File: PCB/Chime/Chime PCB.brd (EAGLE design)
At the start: 99 x 78.9 mm, 33 parts, among them U1 MS5803-02BA, X4 BQ24074

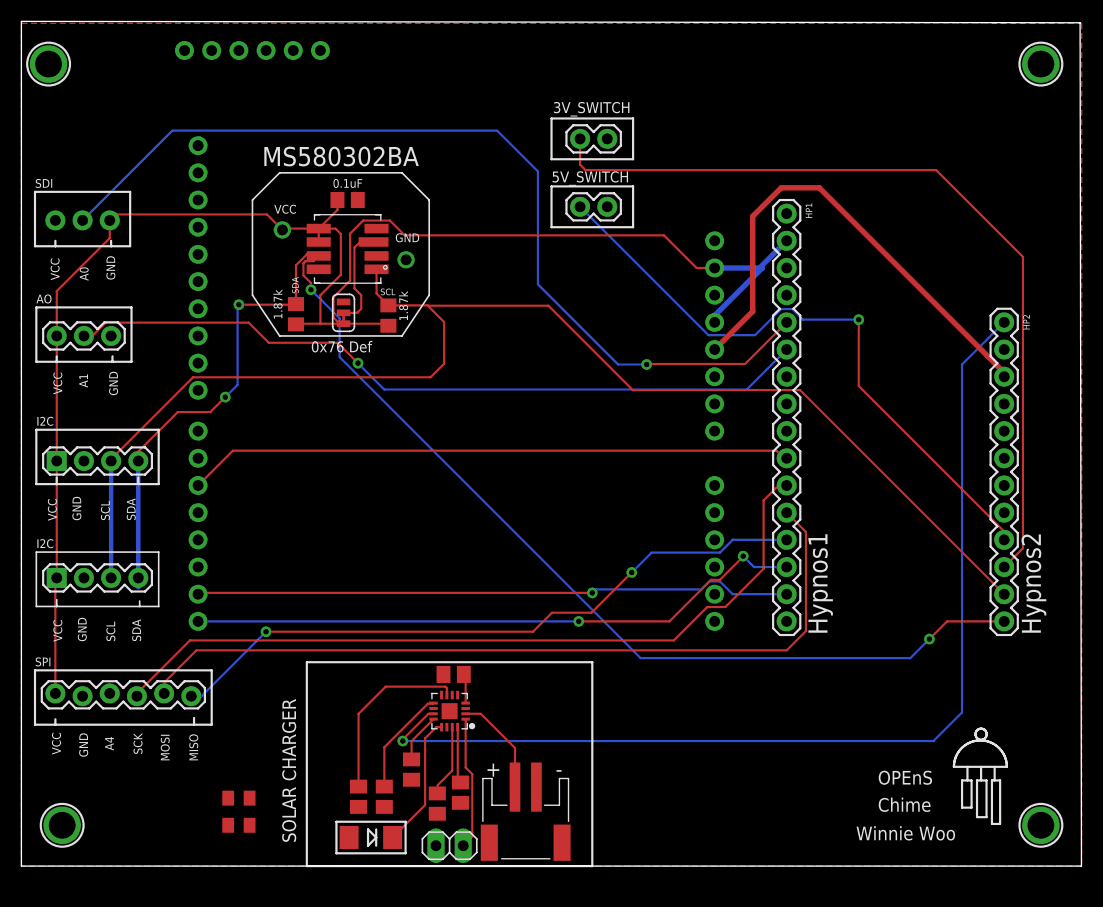
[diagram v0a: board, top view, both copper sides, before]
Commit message: Add files via upload
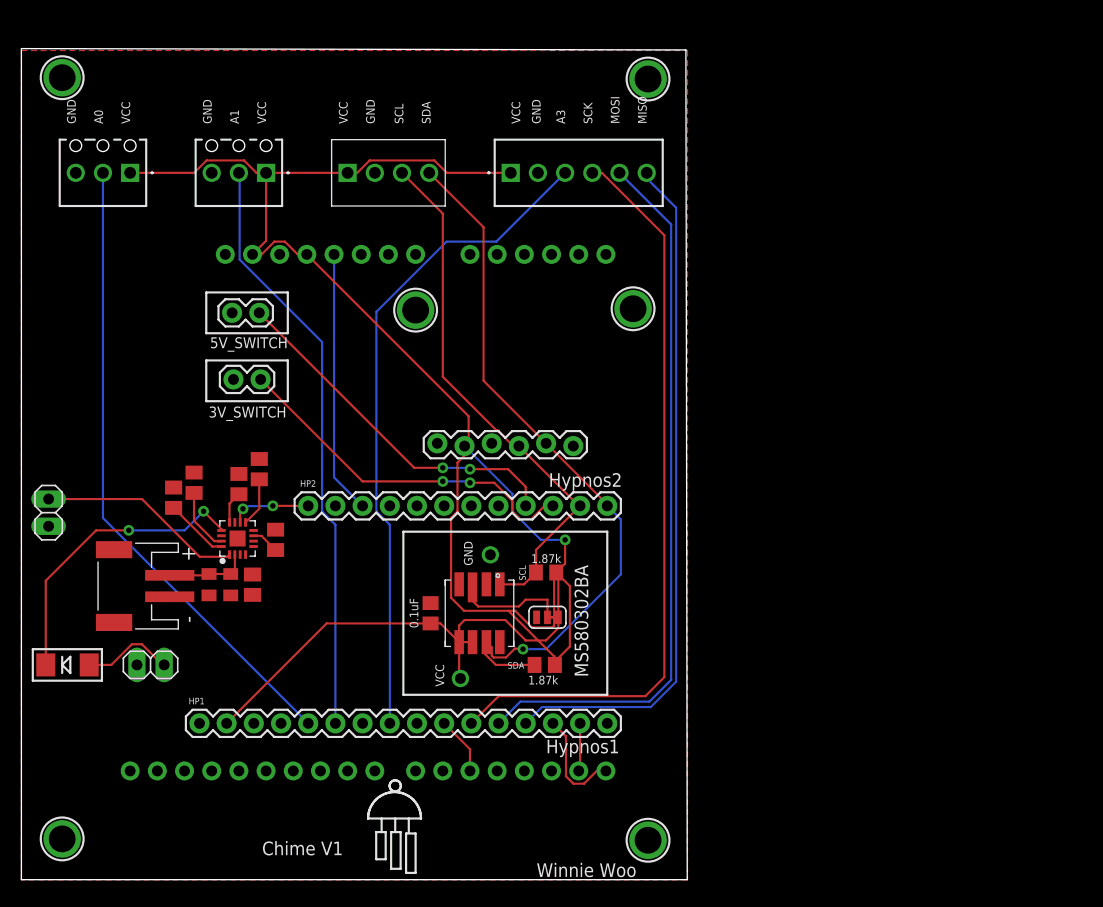
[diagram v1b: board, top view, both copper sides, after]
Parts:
- removed J1_I2C: (no value), SparkFun-Connectors:1X04
- removed J3_AO, J4_SD1: (no value), SparkFun-Connectors:1X03
- removed J6_SPI: (no value), SparkFun-Connectors:1X06_LOCK
- added J1_SPI: 1725698, 1725698:1725698
- added J4_A1, J5_A0: 1725669, 1725669:1725669
- added J6_TSL2591: (no value), SparkFun-Connectors:1X06_LOCK
- added JP9: (no value), pinhead:1X02
- added U$17, U$19: MOUNTINGHOLE2.5, microbuilder:MOUNTINGHOLE_2.5_PLATED
- J2_I2C: value (none) -> 1725672; device SparkFun-Connectors:1X04 -> 1725672:1725672
- U$1: device LTE_BOARD:LTE_BOARD_FOOTPRINT -> LTE_BOARD_LOOM:LTE_BOARD_FOOTPRINT
- moved HP1 72.7 mm to (16.6, 14.6), turned to 0 degrees
- moved HP2 67.2 mm to (26.8, 34.9), turned to 0 degrees
- moved JP8 48.7 mm to (2.54, 34.3), turned to 270 degrees
- moved U$1 45.7 mm to (19.1, 58.4), turned to 180 degrees
- moved JP4 45.1 mm to (41.0, 18.8), turned to 90 degrees
- moved BATT 43.3 mm to (10.2, 27.4), turned to 90 degrees
- moved R1 40.2 mm to (48.9, 20.1), turned to 0 degrees
- moved C1 39.4 mm to (38.2, 24.9), turned to 90 degrees
- moved R9 38.4 mm to (14.2, 35.7), turned to 90 degrees
- moved J2_I2C 38.3 mm to (30.5, 66.0)
- moved R4 37.6 mm to (16.1, 37.1), turned to 90 degrees
- moved J7_S3V 37.4 mm to (22.4, 46.7), turned to 180 degrees
- moved U$4 36.7 mm to (58.5, 74.8)
- moved U$5 36.7 mm to (58.5, 3.68)
- moved U1 36.2 mm to (42.8, 24.9), turned to 90 degrees
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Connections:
- removed net A4: J6_SPI.3
- new net INT: J6_TSL2591.6
- new net VIN: J6_TSL2591.1
- net A0: now also J5_A0.2; no longer J4_SD1.2
- net A1: now also J4_A1.2; no longer J3_AO.2
- net A3: now also J1_SPI.3
- net CHARGER_IN: now also JP9.1
- net GND: now also C5.2, C6.2, J1_SPI.2, J4_A1.3, J5_A0.3, J6_TSL2591.3; no longer J1_I2C.2, J3_AO.3, J4_SD1.3, J6_SPI.2
- net MISO: now also J1_SPI.6; no longer J6_SPI.6
- net MOSI: now also J1_SPI.5; no longer J6_SPI.5
- net SCK: now also J1_SPI.4; no longer J6_SPI.4
- net SCL: now also J6_TSL2591.4; no longer J1_I2C.3
- net SDA: now also J6_TSL2591.5; no longer J1_I2C.4
- net VCC: now also J1_SPI.1, J4_A1.1, J5_A0.1, J6_TSL2591.2; no longer J1_I2C.1, J3_AO.1, J4_SD1.1, J6_SPI.1
- net VLIPO: now also C5.1, C6.1
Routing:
- net VBAT: track 95.4 -> 7.59 mm, vias 1 -> 2
- net SCL: track 124.5 -> 50.2 mm
- net SDA: track 130.7 -> 68.1 mm, vias 4 -> 1
- net A3: track 0.00 -> 62.0 mm
- net 4GONOFF: track 57.1 -> 5.44 mm
- net TX: track 56.1 -> 4.50 mm, vias 1 -> 0
- net RX: track 58.0 -> 9.96 mm, vias 2 -> 0
- net 3VSWITCH: track 77.1 -> 33.9 mm, vias 0 -> 2
- net VCC: track 152.2 -> 189.4 mm, vias 0 -> 1
- net A0: track 86.1 -> 59.4 mm, vias 1 -> 0
- net 5VSWITCH: track 58.6 -> 33.4 mm, vias 1 -> 2
- net 5VRAIL: track 46.1 -> 24.6 mm
- net N$2: track 12.5 -> 27.8 mm, vias 0 -> 2
- net A1: track 70.3 -> 55.2 mm, vias 1 -> 0
- net !PGOOD: track 16.8 -> 2.61 mm
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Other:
- board size 99 x 78.9 mm -> 62.2 x 77.6 mm
- board text added: "A3"
- board text added: "Chime V1"
- board text added: "LTE board this side"
- board text removed: "0x76 Def"
- board text removed: "A4"
- board text removed: "AO"
- board text removed: "Chime"
- board text removed: "I2C"
- board text removed: "LTE BOARD this side"
- board text removed: "OPEnS"
- board text removed: "SDI"
- board text removed: "SOLAR CHARGER"
- board text removed: "SPI"
